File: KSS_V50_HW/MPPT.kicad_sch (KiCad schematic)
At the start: 33 parts, among them Q5 DMG3414U-7, U1 SPV1040, U2 INA236

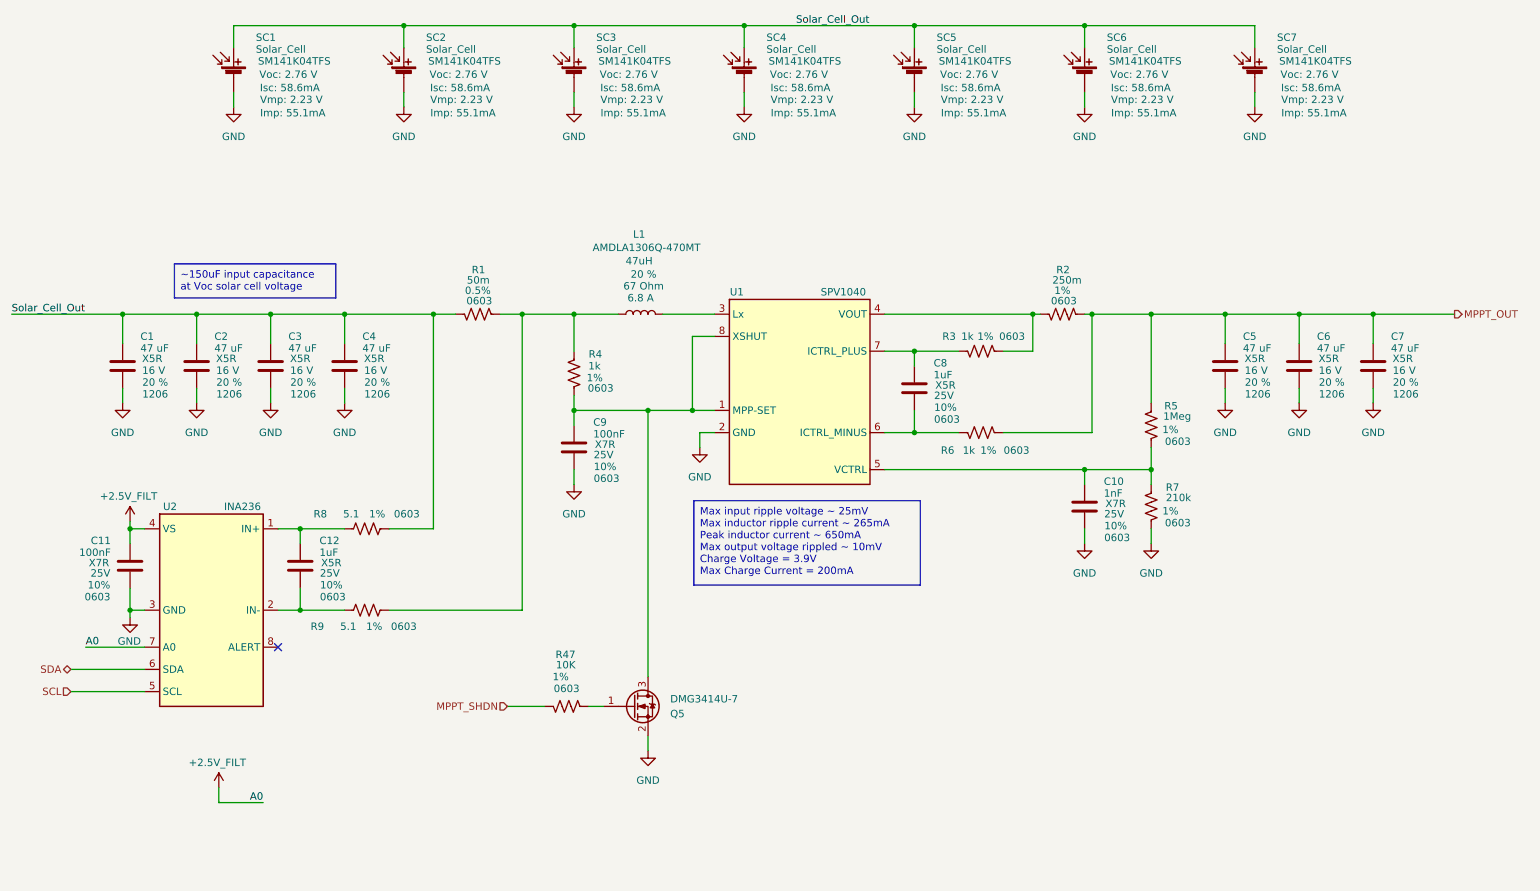
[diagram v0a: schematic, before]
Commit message: post assembly commit
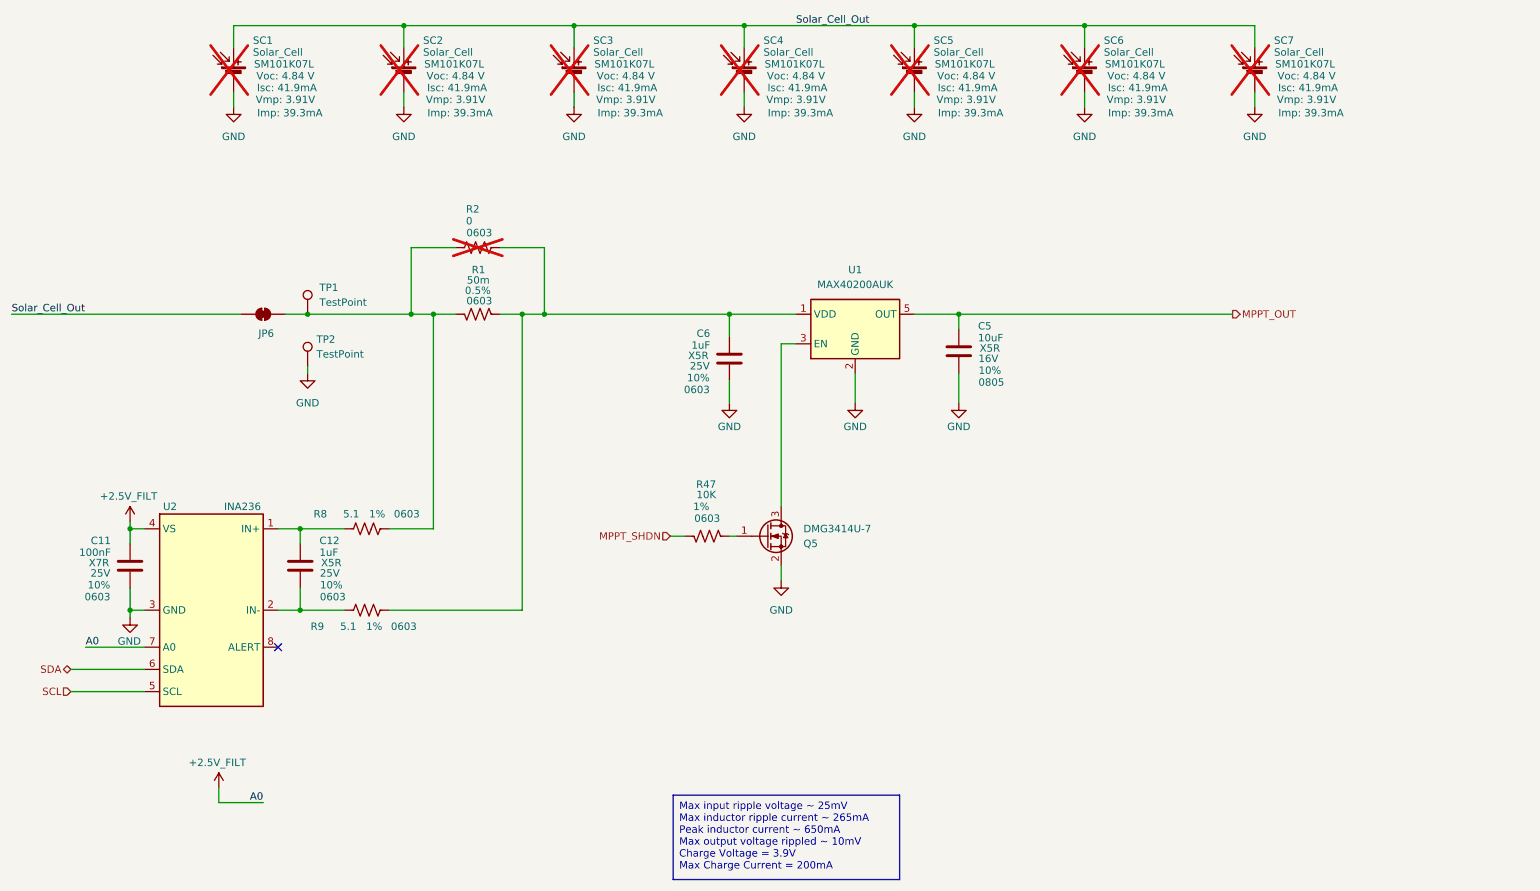
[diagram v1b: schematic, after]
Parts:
- removed C1, C2, C3, C4, C7: 47 uF, Capacitor_SMD:C_1206_3216Metric, symbol Device:C
- removed C10: 1nF, Capacitor_SMD:C_0603_1608Metric, symbol Device:C
- removed C8: 1uF, Capacitor_SMD:C_0603_1608Metric, symbol Device:C
- removed C9: 100nF, Capacitor_SMD:C_0603_1608Metric, symbol Device:C
- removed L1: 47uH, ap_built:AMDLA1306Q-470MT, symbol Device:L
- removed R3, R4, R6: 1k, Resistor_SMD:R_0603_1608Metric, symbol Device:R_US
- removed R5: 1Meg, Resistor_SMD:R_0603_1608Metric, symbol Device:R_US
- removed R7: 210k, Resistor_SMD:R_0603_1608Metric, symbol Device:R_US
- removed U1: SPV1040, Package_SO:TSSOP-8_4.4x3mm_P0.65mm, symbol ap_built:SPV1040
- added JP6: SolderJumper_2_Bridged, Jumper:SolderJumper-2_P1.3mm_Open_TrianglePad1.0x1.5mm, symbol Jumper:SolderJumper_2_Bridged
- added TP1, TP2: TestPoint, TestPoint:TestPoint_Pad_1.5x1.5mm, symbol Connector:TestPoint
- added U1: MAX40200AUK, Package_TO_SOT_SMD:SOT-23-5, symbol Analog_Switch:MAX40200AUK
- C11: JLC_PN (none) -> C92490
- C12: JLC_PN (none) -> C14664
- C5: value 47 uF -> 10uF; footprint Capacitor_SMD:C_1206_3216Metric -> Capacitor_SMD:C_0805_2012Metric; DPN 490-GRM31CR61C476ME44LCT-ND -> 490-6473-1-ND; JLC_PN (none) -> C237493; MPN GRM31CR61C476ME44L -> GRM21BR61C106KE15K; Package 1206 -> 0805; Tolerance 20 % -> 10%; Voltage Rating 16 V -> 16V
- C6: value 47 uF -> 1uF; footprint Capacitor_SMD:C_1206_3216Metric -> Capacitor_SMD:C_0603_1608Metric; DPN 490-GRM31CR61C476ME44LCT-ND -> 311-1445-1-ND; JLC_PN (none) -> C14664; MPN GRM31CR61C476ME44L -> CC0603KRX5R8BB105; Package 1206 -> 0603; Tolerance 20 % -> 10%; Voltage Rating 16 V -> 25V
- Q5: JLC_PN (none) -> C260927
- R1: JLC_PN (none) -> C5372686
- R2: value 250m -> 0; DPN CSR0603FKR250CT-ND -> (none); MPN CSR0603FKR250 -> (none); Tolerance 1% -> (none); now not fitted
- R47: JLC_PN (none) -> C116677
- R8, R9: JLC_PN (none) -> C114626
- SC1, SC2, SC3, SC4, SC5, SC6, SC7: footprint ap_built:SM141K04TFS -> ap_built:SM101K07L; Imp 55.1mA -> 39.3mA; Isc 58.6mA -> 41.9mA; MPN SM141K04TFS -> SM101K07L; Vmp 2.23 V -> 3.91V; Voc 2.76 V -> 4.84 V; now not fitted
- U2: JLC_PN (none) -> C5443912
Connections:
- net GND: now also TP2.1, U1.2 (GND)
- net MPPT_OUT: now also U1.5 (OUT); no longer C6.1, R2.2
- net Solar_Cell_Out: now also JP6.1 (A); no longer R1.1, R8.1
- net at R2.1: now also C6.1, R1.2, R9.1, U1.1 (VDD)
- net at Q5.3 (D): now also U1.3 (EN)
- new net: JP6.2 (B), R1.1, R2.2, R8.1, TP1.1
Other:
- moved on the sheet: Q5, R47
